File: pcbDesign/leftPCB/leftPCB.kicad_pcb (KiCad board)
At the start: 2 copper layers, 57.5 x 90 mm, 22 parts, among them J1 Conn_01x12_Pin, J2 Conn_01x07_Pin, J3 Conn_01x01_Pin, J4 Conn_01x01_Pin, J5 440055-2, SW1 UP, SW2 DOWN, SW3 LEFT, SW4 RIGHT, SW5 RotaryEncoder

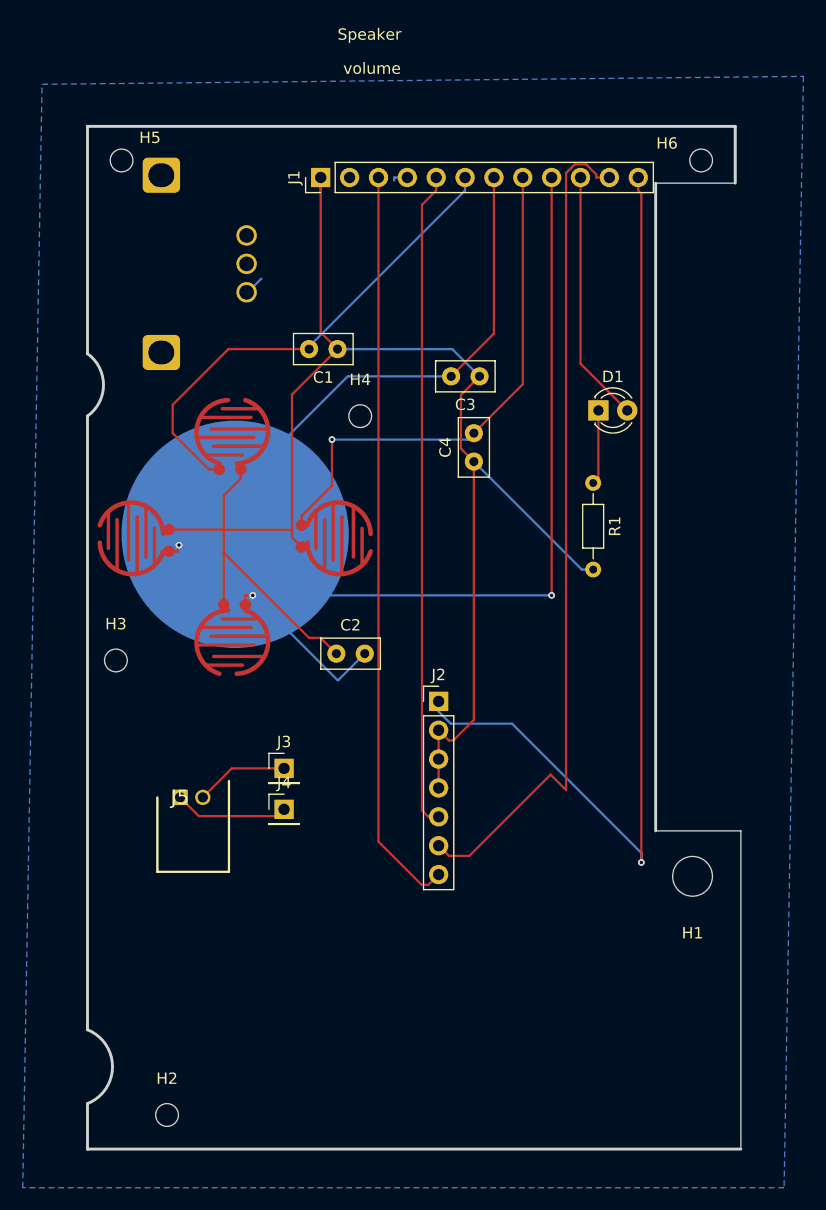
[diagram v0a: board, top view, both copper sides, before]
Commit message: rerouted
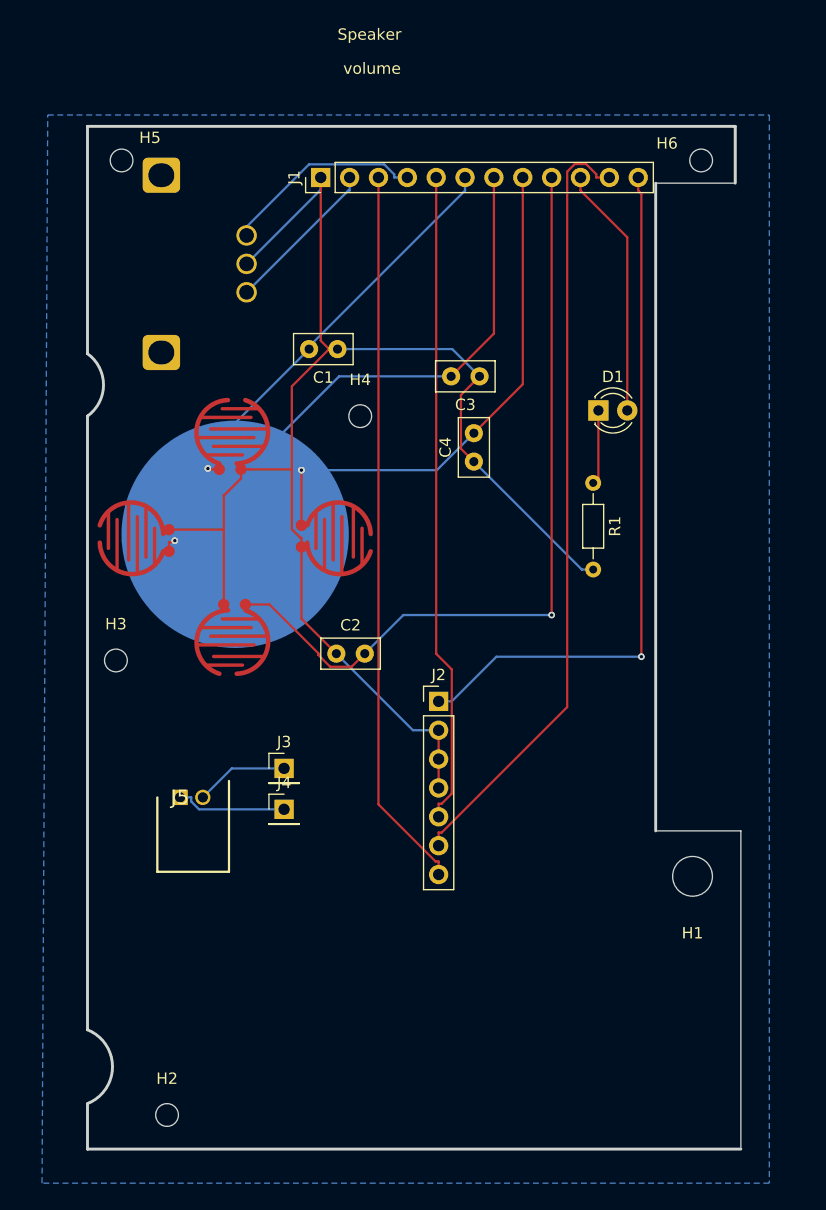
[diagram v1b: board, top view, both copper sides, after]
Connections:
- SW2 pad 1: /Down -> GND
- SW2 pad 2: GND -> /Down
- SW3 pad 1: (no net) -> GND
- SW3 pad 2: (no net) -> /Left
- SW4 pad 1: (no net) -> GND
- SW4 pad 2: (no net) -> /Right
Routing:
- net /5v: track 85.1 -> 61.8 mm
- net /Volume_A: track 1.42 -> 17.8 mm
- net /Volume_B: track 1.80 -> 13.9 mm
- net GND: track 142.7 -> 131.6 mm
- net /Down: track 78.4 -> 69.7 mm, vias 2 -> 1
- net /Up: track 42.7 -> 36.0 mm, vias 0 -> 1
- net /Clk: track 74.2 -> 68.8 mm
- net /LR_Clk: track 65.7 -> 63.7 mm
